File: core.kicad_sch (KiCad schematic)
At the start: 41 parts, among them U1 ESP32-P4, U2 W25Q128JVS, Y1 40MHz 10ppm, Y2 32.768k

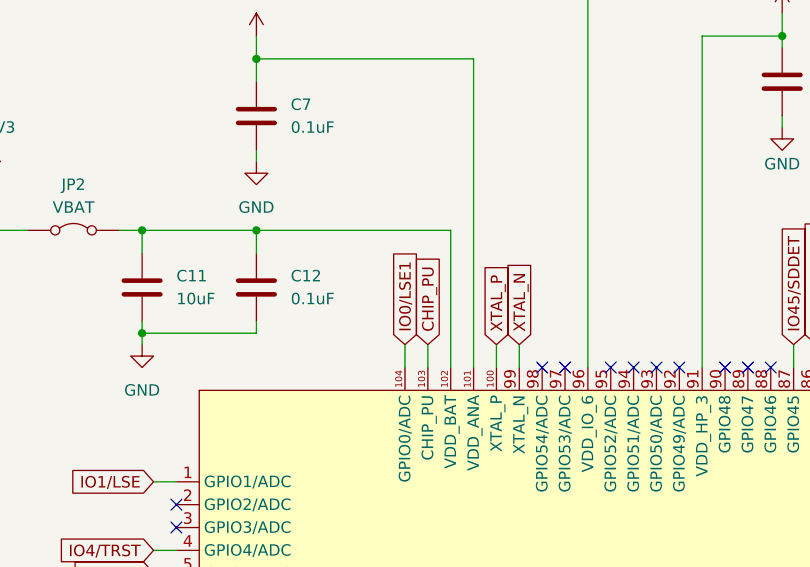
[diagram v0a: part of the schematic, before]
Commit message: Typo fix
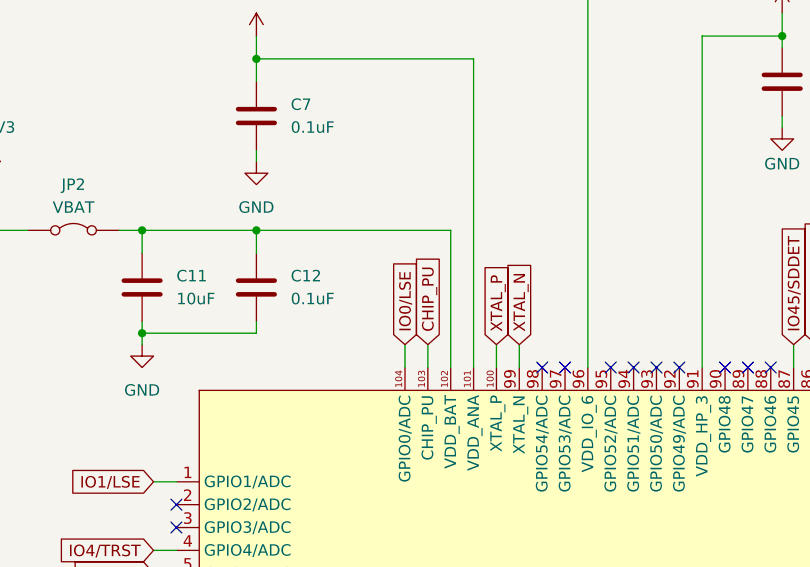
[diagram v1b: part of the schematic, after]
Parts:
- U1: footprint PCM_Espressif:ESP32-P4 -> Espressif:ESP32-P4
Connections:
- net IO0/LSE1 is gone; now on net IO0/LSE: U1.104 (GPIO0/ADC)
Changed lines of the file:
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@@
 		)
 	)
-	(global_label "IO0{slash}LSE1"
+	(global_label "IO0{slash}LSE"
 		(shape input)
 		(at 144.78 96.52 90)
@@
 		)
 		(property "Intersheetrefs" "${INTERSHEET_REFS}"
-			(at 144.78 87.85 90)
+			(at 144.78 85.6729 90)
 			(effects
 				(font
@@
 			)
 		)
-		(property "Footprint" "PCM_Espressif:ESP32-P4"
+		(property "Footprint" "Espressif:ESP32-P4"
 			(at 121.92 185.42 0)
 			(effects

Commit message: Assign footprint
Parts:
- C11, C14, C17, C18, C19, C20, C22, C27, C28, C30, C34: footprint Capacitor_SMD:C_0603_1608Metric -> Capacitor_SMD:C_0402_1005Metric
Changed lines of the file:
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@@
 			)
 		)
-		(property "Footprint" "Capacitor_SMD:C_0603_1608Metric"
+		(property "Footprint" "Capacitor_SMD:C_0402_1005Metric"
 			(at 336.2452 96.52 0)
 			(effects
@@
 			)
 		)
-		(property "Footprint" "Capacitor_SMD:C_0603_1608Metric"
+		(property "Footprint" "Capacitor_SMD:C_0402_1005Metric"
 			(at 101.2952 184.15 0)
 			(effects
@@
 			)
 		)
-		(property "Footprint" "Capacitor_SMD:C_0603_1608Metric"
+		(property "Footprint" "Capacitor_SMD:C_0402_1005Metric"
 			(at 116.5352 93.98 0)
 			(effects
@@
 			)
 		)
-		(property "Footprint" "Capacitor_SMD:C_0603_1608Metric"
+		(property "Footprint" "Capacitor_SMD:C_0402_1005Metric"
 			(at 319.7352 96.52 0)
 			(effects
@@
 			)
 		)
-		(property "Footprint" "Capacitor_SMD:C_0603_1608Metric"
+		(property "Footprint" "Capacitor_SMD:C_0402_1005Metric"
 			(at 267.6652 167.64 0)
 			(effects
@@
 			)
 		)
-		(property "Footprint" "Capacitor_SMD:C_0603_1608Metric"
+		(property "Footprint" "Capacitor_SMD:C_0402_1005Metric"
 			(at 82.2452 140.97 0)
 			(effects
@@
 			)
 		)
-		(property "Footprint" "Capacitor_SMD:C_0603_1608Metric"
+		(property "Footprint" "Capacitor_SMD:C_0402_1005Metric"
 			(at 270.2052 96.52 0)
 			(effects
@@
 			)
 		)
-		(property "Footprint" "Capacitor_SMD:C_0603_1608Metric"
+		(property "Footprint" "Capacitor_SMD:C_0402_1005Metric"
 			(at 357.8352 96.52 0)
 			(effects
@@
 			)
 		)
-		(property "Footprint" "Capacitor_SMD:C_0603_1608Metric"
+		(property "Footprint" "Capacitor_SMD:C_0402_1005Metric"
 			(at 347.6752 96.52 0)
 			(effects
@@
 			)
 		)
-		(property "Footprint" "Capacitor_SMD:C_0603_1608Metric"
+		(property "Footprint" "Capacitor_SMD:C_0402_1005Metric"
 			(at 265.1252 223.52 0)
 			(effects
@@
 			)
 		)
-		(property "Footprint" "Capacitor_SMD:C_0603_1608Metric"
+		(property "Footprint" "Capacitor_SMD:C_0402_1005Metric"
 			(at 120.3452 214.63 0)
 			(effects
